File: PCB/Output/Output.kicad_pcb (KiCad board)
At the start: 2 copper layers, 47.7 x 34.3 mm, 39 parts, among them J1 USB-C, J10 O8, J11 O9, J12 O10, J2 POWER, J3 O1, J4 O2, J5 O3, J6 O4, J7 O5, J8 O6, J9 O7, U1 ESP32-PICO-MINI-02, U10 QR, U11 CH340X, U3 ISL89410, U4 ISL89410, U5 ISL89410, U6 ISL89410, U7 ISL89410, U8 MD8942, U9 AA

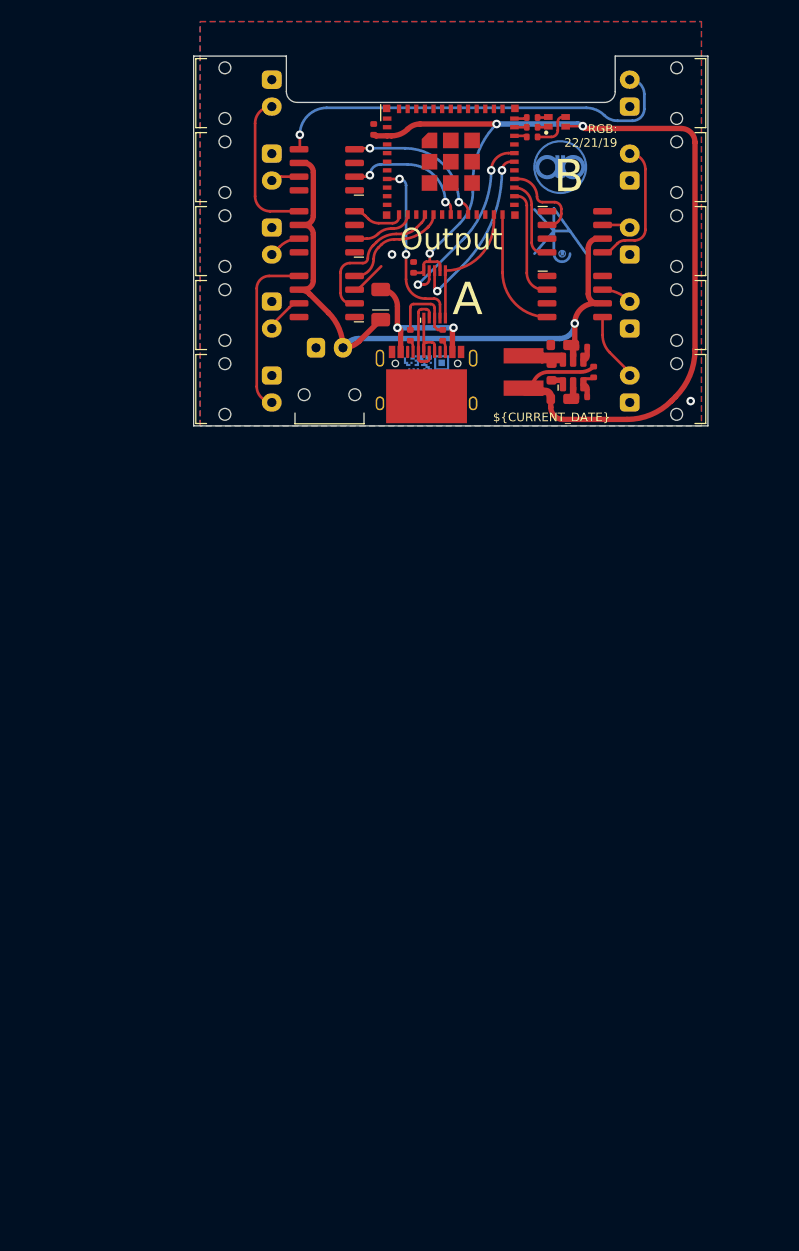
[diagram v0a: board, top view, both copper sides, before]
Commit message: Panel
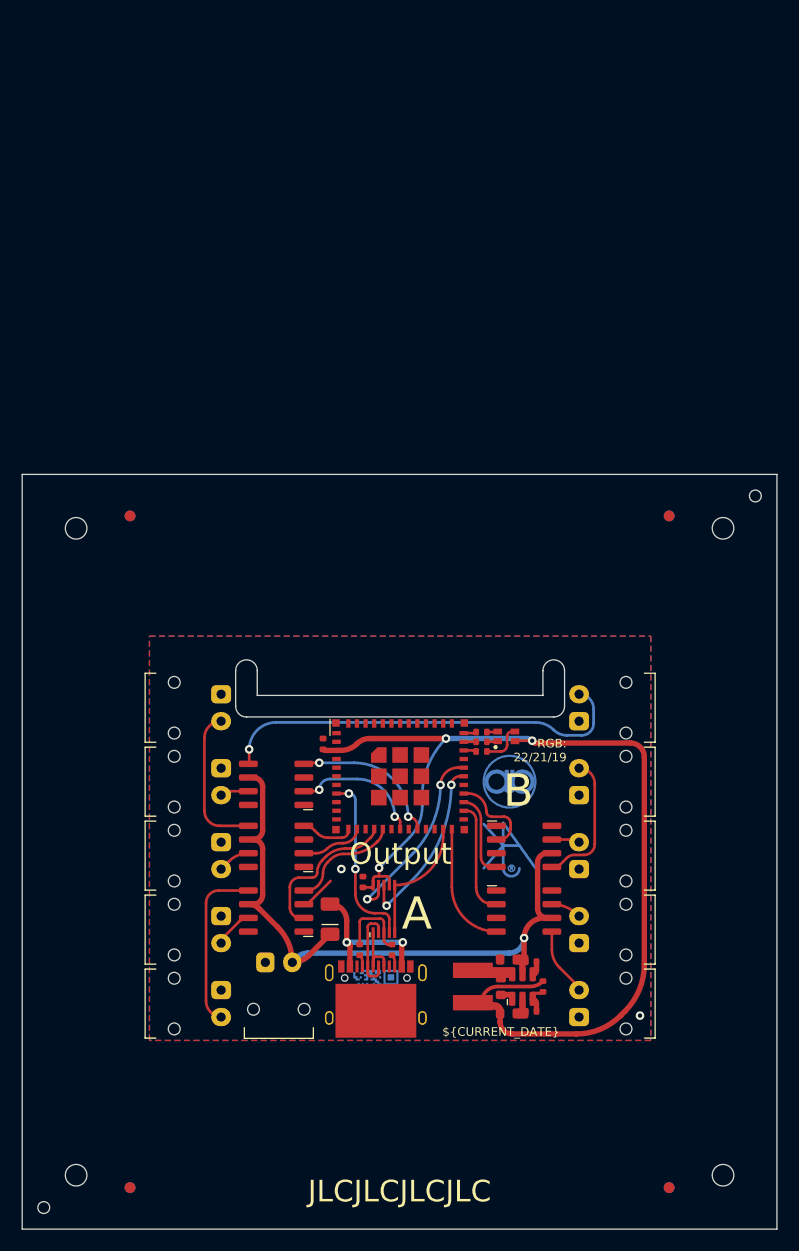
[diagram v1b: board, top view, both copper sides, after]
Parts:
- added PCB1: 70x70, RevK:PCB7070, F.Cu at (100.0, 100.0)
- added V1: ~, RevK:VCUT70, F.Cu at (100.0, 83.2)
- added V2: ~, RevK:VCUT70, F.Cu at (100.0, 117.5)
- added V3: ~, RevK:VCUT70, B.Cu at (76.2, 100.0)
- added V4: ~, RevK:VCUT70, B.Cu at (123.9, 100.0)
- moved R12 57.2 mm to (107.6, 88.9)
- moved AJK1 57.2 mm to (109.6, 99.4)
- moved C1 57.2 mm to (92.9, 90.0)
- moved C2 57.2 mm to (96.6, 102.8)
- moved C3 57.2 mm to (110.1, 110.0)
- moved C4 57.2 mm to (110.1, 115.0)
- moved C9 57.2 mm to (109.4, 112.5)
- moved D2 57.2 mm to (93.5, 106.2)
- moved D3 57.2 mm to (109.9, 89.3)
- moved J10 57.2 mm to (116.7, 93.5)
- moved J11 57.2 mm to (116.7, 86.6)
- moved J12 57.2 mm to (83.5, 93.5)
- moved J3 57.2 mm to (83.5, 86.6)
- moved J4 57.2 mm to (83.5, 100.4)
- moved J5 57.2 mm to (83.5, 114.1)
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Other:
- board size 47.7 x 34.3 mm -> 70 x 70 mm
